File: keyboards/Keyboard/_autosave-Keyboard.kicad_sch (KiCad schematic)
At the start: 92 parts

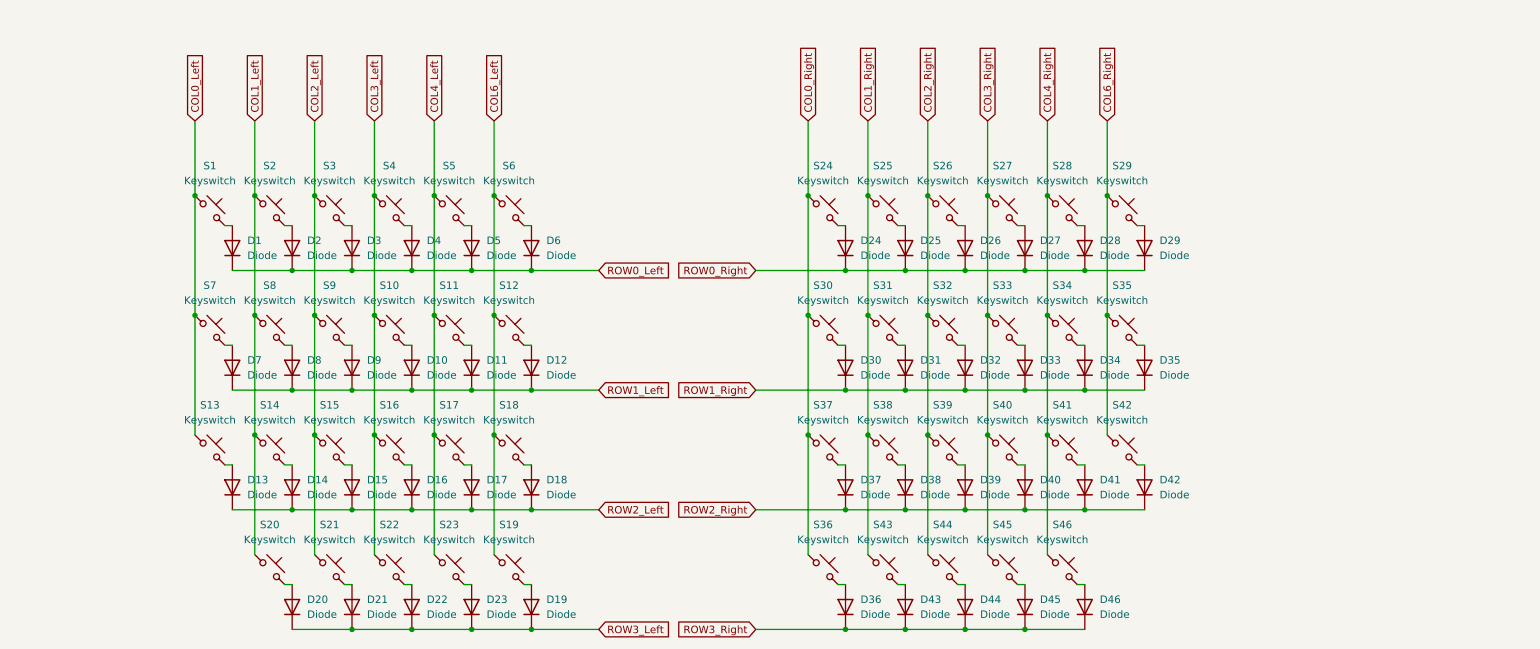
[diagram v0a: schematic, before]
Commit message: added backupfiles and contents
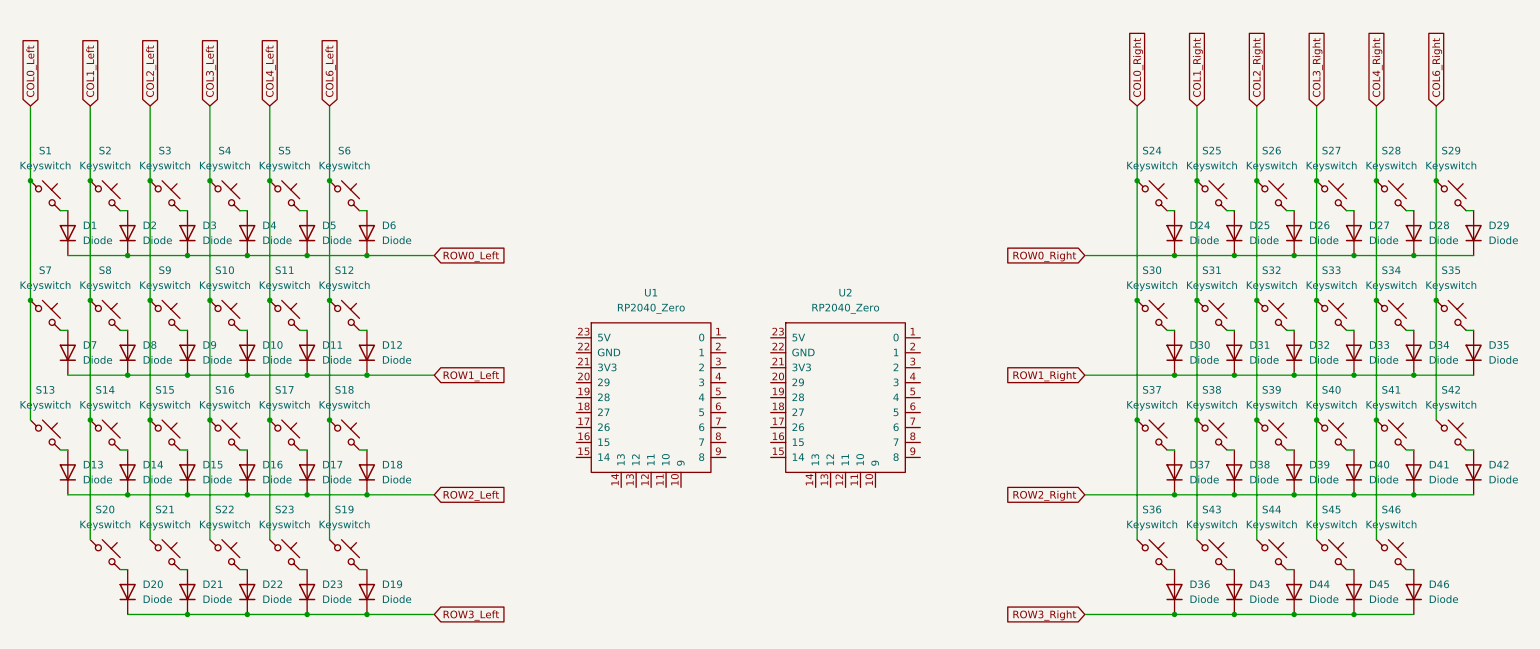
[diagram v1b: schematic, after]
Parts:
- added U1, U2: RP2040_Zero, ScottoKeebs_MCU:RP2040_Zero, symbol ScottoKeebs:MCU_RP2040_Zero
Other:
- moved on the sheet: D1, D10, D11, D12, D13, D14, D15, D16, D17, D18, D19, D2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
